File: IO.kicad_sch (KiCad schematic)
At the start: 18 parts, among them Q4 S8050, Q5 IRF3708S, U13 LTV-817S, U14 LTV-817S

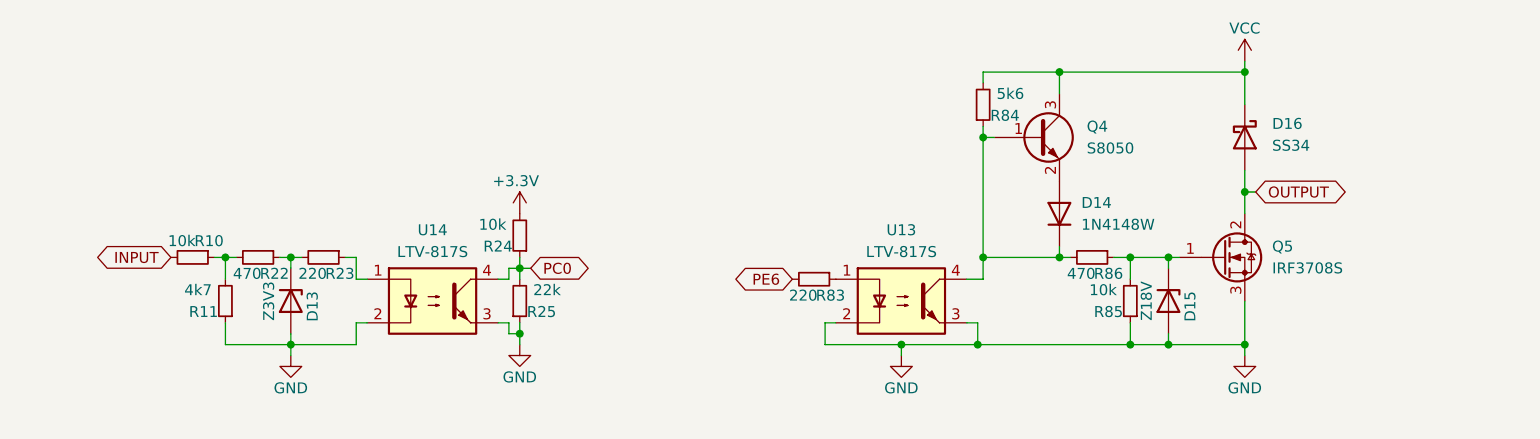
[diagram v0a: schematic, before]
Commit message: Add files via upload
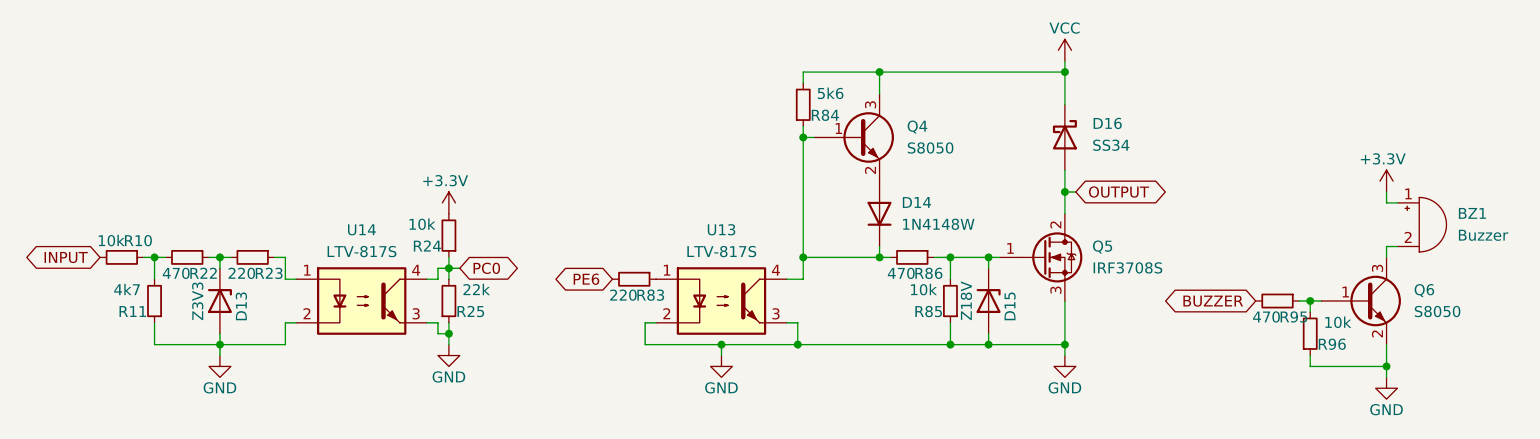
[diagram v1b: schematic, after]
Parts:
- added BZ1: Buzzer, Buzzer_Beeper:MagneticBuzzer_PUI_AT-0927-TT-6-R, symbol Device:Buzzer
- added Q6: S8050, Package_TO_SOT_SMD:SOT-23, symbol Transistor_BJT:BC847
- added R95: 470, Resistor_SMD:R_0603_1608Metric, symbol Device:R_Small
- added R96: 10k, Resistor_SMD:R_0603_1608Metric, symbol Device:R_Small
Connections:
- net +3.3V: now also BZ1.1 (-)
- net GND: now also Q6.2 (E), R96.1
- new net: Q6.1 (B), R95.1, R96.2
- new net: BZ1.2 (+), Q6.3 (C)
- new net BUZZER: R95.2
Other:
- moved on the sheet: D13, D14, D15, D16, Q4, Q5, R10, R11, R22, R23, R24, R25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
